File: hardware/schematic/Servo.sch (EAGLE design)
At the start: 23 parts

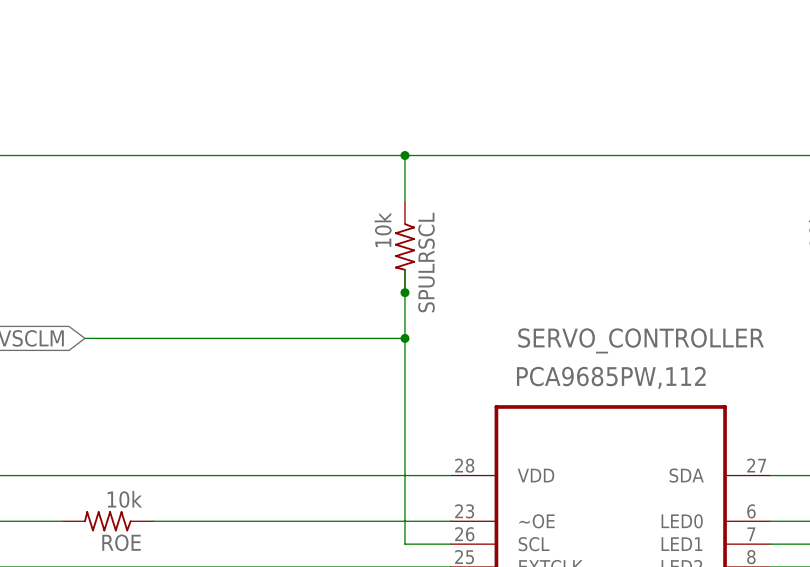
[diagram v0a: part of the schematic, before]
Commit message: Update Servo.sch
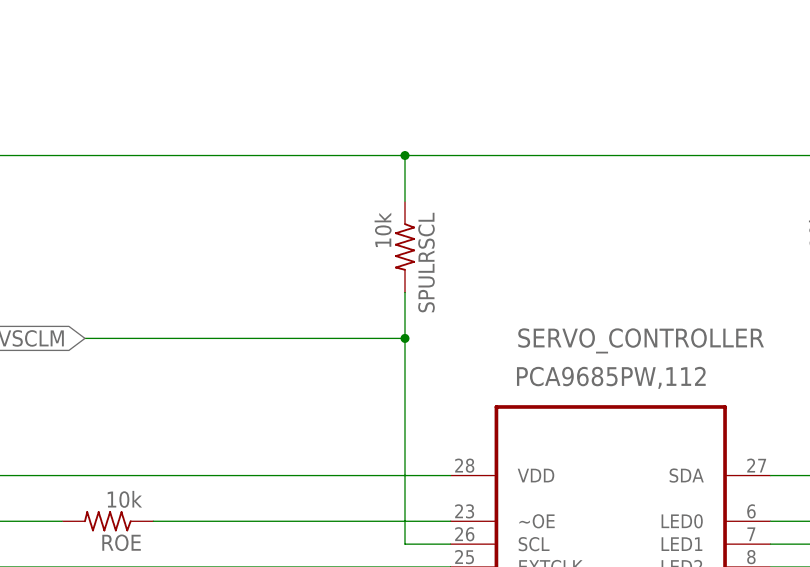
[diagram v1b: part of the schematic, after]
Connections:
- net N$39 renamed OE
- net N$44 renamed A1
- net N$45 renamed A0
- net N$46 renamed A2
- net N$47 renamed A3
- net N$48 renamed A4
- net N$49 renamed A5
- net N$50 renamed LED_RS6
- net N$64 renamed CC1_RUSB4
- net N$65 renamed CC2
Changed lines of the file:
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@@
 </segment>
 </net>
-<net name="N$39" class="0">
+<net name="OE" class="0">
 <segment>
 <pinref part="SERVO_CONTROLLER" gate="A" pin="~OE"/>
@@
 </segment>
 </net>
-<net name="N$45" class="0">
+<net name="A0" class="0">
 <segment>
 <pinref part="SERVO_CONTROLLER" gate="A" pin="A0"/>
@@
 </segment>
 </net>
-<net name="N$44" class="0">
+<net name="A1" class="0">
 <segment>
 <pinref part="SERVO_CONTROLLER" gate="A" pin="A1"/>
@@
 </segment>
 </net>
-<net name="N$46" class="0">
+<net name="A2" class="0">
 <segment>
 <pinref part="SERVO_CONTROLLER" gate="A" pin="A2"/>
@@
 </segment>
 </net>
-<net name="N$47" class="0">
+<net name="A3" class="0">
 <segment>
 <pinref part="SERVO_CONTROLLER" gate="A" pin="A3"/>
@@
 </segment>
 </net>
-<net name="N$48" class="0">
+<net name="A4" class="0">
 <segment>
 <pinref part="SERVO_CONTROLLER" gate="A" pin="A4"/>
@@
 </segment>
 </net>
-<net name="N$49" class="0">
+<net name="A5" class="0">
 <segment>
 <pinref part="SERVO_CONTROLLER" gate="A" pin="A5"/>
@@
 </segment>
 </net>
-<net name="N$50" class="0">
+<net name="LED_RS6" class="0">
 <segment>
 <pinref part="LED4" gate="G$1" pin="C"/>
@@
 <pinref part="SPULRSCL" gate="G$1" pin="2"/>
 <wire x1="83.82" y1="111.76" x2="83.82" y2="116.84" width="0.1524" layer="91"/>
-<wire x1="83.82" y1="116.84" x2="83.82" y2="119.38" width="0.1524" layer="91"/>
-<junction x="83.82" y="116.84"/>
 <wire x1="83.82" y1="111.76" x2="48.26" y2="111.76" width="0.1524" layer="91"/>
 <junction x="83.82" y="111.76"/>
@@
 </segment>
 </net>
-<net name="N$64" class="0">
+<net name="CC1_RUSB4" class="0">
 <segment>
 <pinref part="I2C_USBC_OUT" gate="A" pin="CC1"/>
@@
 </segment>
 </net>
-<net name="N$65" class="0">
+<net name="CC2" class="0">
 <segment>
 <pinref part="I2C_USBC_OUT" gate="A" pin="CC2"/>
